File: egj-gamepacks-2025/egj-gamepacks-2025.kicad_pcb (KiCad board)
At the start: 2 copper layers, 52.3 x 64 mm, 81 parts, among them J1 USB_B_Micro, J2 Conn_01x03_Pin, J5 GameBoy_GamePak_AGB-002, SW1 SW_Push, SW2 SW_Push, U1 W25Q128JVS, U10 SP3012-06UTG, U11 VL6180XV0NR_1, U12 TXS0108EPW, U13 LD1117S18TR_SOT223, U14 BNO055, U15 SP3012-06UTG, U2 DNF, U3 NCP1117-3.3_SOT223, U4 RP2350_80QFN, U5 USBLC6-2P6, U6 SP3012-06UTG, U7 SP3012-06UTG, U8 SP3012-06UTG, U9 SP3012-06UTG, Y1 ABM8-272-T3

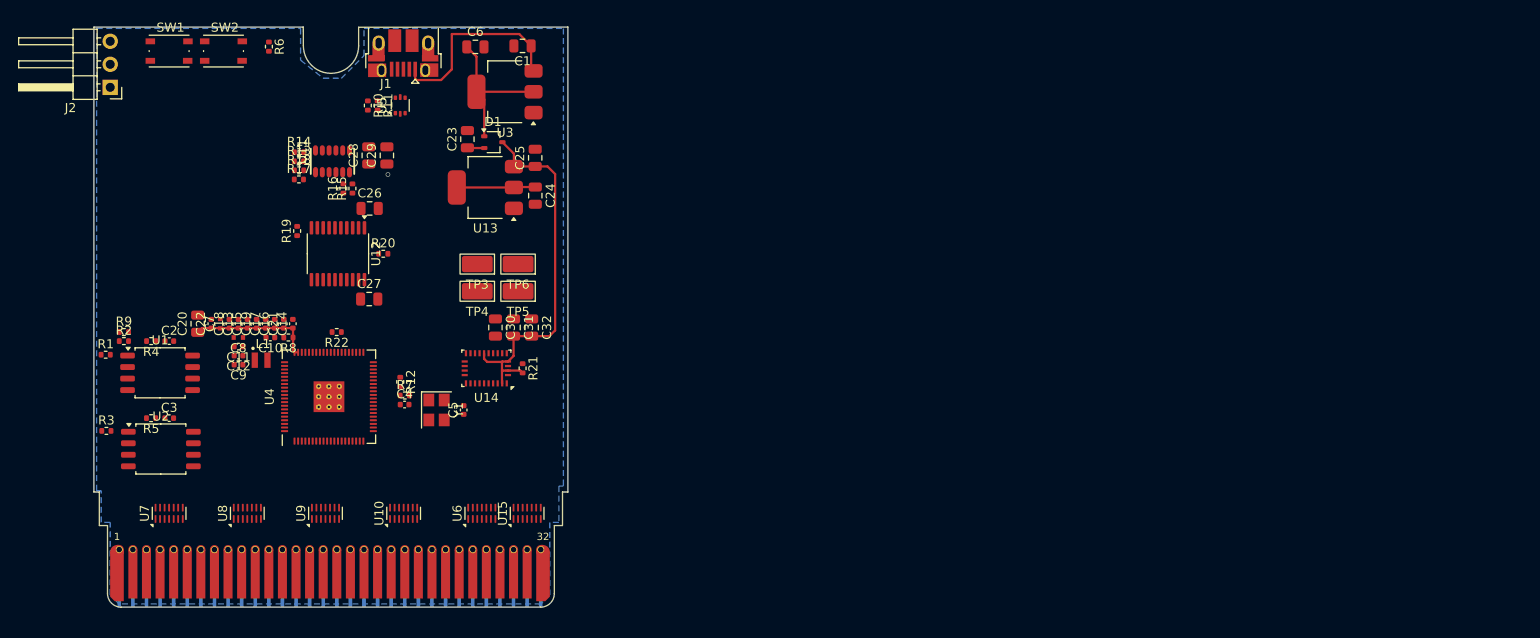
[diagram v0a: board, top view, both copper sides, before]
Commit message: UPDATE: sync local schematic and board work
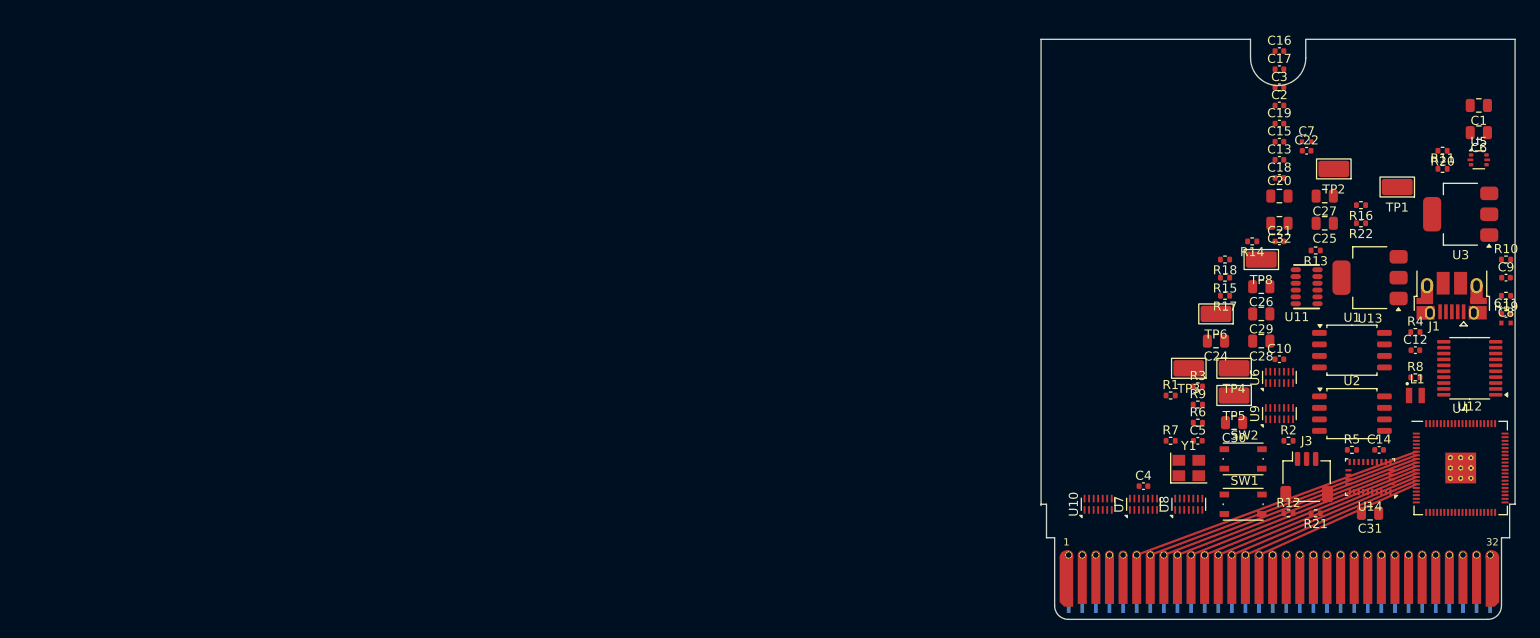
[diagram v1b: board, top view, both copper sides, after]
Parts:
- removed C23: 100u, Capacitor_SMD:C_0805_2012Metric
- removed D1: BAT54CW, Package_TO_SOT_SMD:SOT-323_SC-70
- removed J2: Conn_01x03_Pin, Connector_PinHeader_2.54mm:PinHeader_1x03_P2.54mm_Horizontal
- removed U15: SP3012-06UTG, Package_DFN_QFN:DFN-14_1.35x3.5mm_P0.5mm
- added J3: SM03B-SRSS-TB, Connector_JST:JST_SH_SM03B-SRSS-TB_1x03-1MP_P1.00mm_Horizontal, F.Cu at (251.0, 109.0)
- added TP1: TestPoint, TestPoint:TestPoint_Keystone_5015_Micro_Mini, F.Cu at (261.0, 77.0)
- added TP2: TestPoint, TestPoint:TestPoint_Keystone_5015_Micro_Mini, F.Cu at (254.0, 75.0)
- added TP8: TestPoint, TestPoint:TestPoint_Keystone_5015_Micro_Mini, F.Cu at (246.0, 85.0)
- U13: value LD1117S18TR_SOT223 -> AP7361C-28E
- moved C9 140.2 mm to (273.0, 87.0), turned to 0 degrees
- moved C11 139.9 mm to (273.0, 91.0), turned to 0 degrees
- moved C8 139.9 mm to (273.0, 92.0), turned to 0 degrees
- moved R4 139.5 mm to (263.0, 93.0), turned to 0 degrees
- moved R19 133.6 mm to (273.0, 89.0), turned to 180 degrees
- moved R5 132.5 mm to (256.0, 106.0), turned to 0 degrees
- moved U1 131.5 mm to (256.0, 95.0)
- moved U2 131.5 mm to (256.0, 102.0)
- moved C12 129.8 mm to (263.0, 95.0), turned to 0 degrees
- moved R2 129.0 mm to (249.0, 105.0)
- moved SW1 128.6 mm to (244.0, 112.0)
- moved C3 127.8 mm to (248.0, 66.0)
- moved L1 127.4 mm to (263.0, 100.0)
- moved R10 126.7 mm to (273.0, 85.0), turned to 0 degrees
- moved U12 125.5 mm to (269.0, 97.0), turned to 180 degrees
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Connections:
- net /RP2350/+1V1 renamed +1V1
- C24 pad 1: +1V8 -> +2V8
- C26 pad 1: +1V8 -> +2V8
- C28 pad 1: +1V8 -> +2V8
- C29 pad 1: +1V8 -> +2V8
- C6 pad 1: +3V3_USB -> +3V3
- R10 pad 1: /Power/USB.USB_D_C+ -> /RP2350/USB_D+
- R11 pad 1: /Power/USB.USB_D_C- -> /RP2350/USB_D-
- R13 pad 1: +1V8 -> +2V8
- R14 pad 1: +1V8 -> +2V8
- R17 pad 1: +1V8 -> +2V8
- R18 pad 1: +1V8 -> +2V8
- U10 pad 1: /GBA_Connector/GBA_ADD13 -> unconnected-(U10-Pad1)
- U10 pad 11: /GBA_Connector/GBA_DATA0 -> /GBA_Connector/GBA_SIG.N_CS
- U10 pad 12: /GBA_Connector/GBA_ADD15 -> /GBA_Connector/GBA_SIG.N_RD
- U10 pad 13: /GBA_Connector/GBA_ADD14 -> /GBA_Connector/GBA_SIG.N_WR
- U10 pad 14: /GBA_Connector/GBA_ADD13 -> /GBA_Connector/GBA_SIG.PHI
- U10 pad 2: /GBA_Connector/GBA_ADD14 -> unconnected-(U10-Pad2)
- U10 pad 3: /GBA_Connector/GBA_ADD15 -> unconnected-(U10-Pad3)
- U10 pad 4: /GBA_Connector/GBA_DATA0 -> unconnected-(U10-Pad4)
- U10 pad 5: GND -> unconnected-(U10-Pad5)
- U10 pad 6: /GBA_Connector/GBA_DATA1 -> unconnected-(U10-Pad6)
- U10 pad 7: /GBA_Connector/GBA_DATA2 -> unconnected-(U10-Pad7)
- U10 pad 8: /GBA_Connector/GBA_DATA2 -> /GBA_Connector/GBA_SIG.IRQ
- U10 pad 9: /GBA_Connector/GBA_DATA1 -> /GBA_Connector/GBA_SIG.N_CS2
- U11 pad 10: +1V8 -> +2V8
- U11 pad 8: +1V8 -> +2V8
- U12 pad 2: +1V8 -> +2V8
- U13 pad 1: GND -> +3V3
- U13 pad 2: +1V8 -> GND
- U13 pad 3: +3V3 -> +2V8
- U3 pad 2: +3V3_USB -> +3V3
- U4 pad 1: /GBA_Connector/GBA_ADD0 -> /GBA_Connector/GBA_DATA4
- U4 pad 11: /GBA_Connector/GBA_ADD8 -> /GBA_Connector/GBA_ADD4
- U4 pad 12: /GBA_Connector/GBA_ADD9 -> /GBA_Connector/GBA_ADD5
- U4 pad 13: /GBA_Connector/GBA_ADD10 -> /GBA_Connector/GBA_ADD6
- U4 pad 14: /GBA_Connector/GBA_ADD11 -> /GBA_Connector/GBA_ADD7
- U4 pad 16: /GBA_Connector/GBA_ADD12 -> /GBA_Connector/GBA_ADD8
- U4 pad 17: /GBA_Connector/GBA_ADD13 -> /GBA_Connector/GBA_ADD9
- U4 pad 18: /GBA_Connector/GBA_ADD14 -> /GBA_Connector/GBA_ADD10
- U4 pad 19: /GBA_Connector/GBA_ADD15 -> /GBA_Connector/GBA_ADD11
- U4 pad 2: /GBA_Connector/GBA_ADD1 -> /GBA_Connector/GBA_DATA5
- U4 pad 20: /GBA_Connector/GBA_DATA0 -> /GBA_Connector/GBA_ADD12
- U4 pad 21: /GBA_Connector/GBA_DATA1 -> /GBA_Connector/GBA_ADD13
- U4 pad 22: /GBA_Connector/GBA_DATA2 -> /GBA_Connector/GBA_ADD14
- U4 pad 23: /GBA_Connector/GBA_DATA3 -> /GBA_Connector/GBA_ADD15
- U4 pad 25: /GBA_Connector/GBA_DATA4 -> /GBA_Connector/GBA_SIG.PHI
- U4 pad 26: /GBA_Connector/GBA_DATA5 -> /GBA_Connector/GBA_SIG.N_WR
- U4 pad 27: /GBA_Connector/GBA_DATA6 -> /GBA_Connector/GBA_SIG.N_RD
- U4 pad 28: /GBA_Connector/GBA_DATA7 -> /GBA_Connector/GBA_SIG.N_CS
- U4 pad 3: /GBA_Connector/GBA_ADD2 -> /GBA_Connector/GBA_DATA6
- U4 pad 4: /GBA_Connector/GBA_ADD3 -> /GBA_Connector/GBA_DATA7
- U4 pad 58: +3V3_USB -> unconnected-(U4-GPIO47_ADC7-Pad58)
- U4 pad 6: /GBA_Connector/GBA_ADD4 -> /GBA_Connector/GBA_ADD0
- U4 pad 7: /GBA_Connector/GBA_ADD5 -> /GBA_Connector/GBA_ADD1
- U4 pad 77: /GBA_Connector/GBA_SIG.PHI -> /GBA_Connector/GBA_DATA0
- U4 pad 78: /GBA_Connector/GBA_SIG.N_WR -> /GBA_Connector/GBA_DATA1
- U4 pad 79: /GBA_Connector/GBA_SIG.N_RD -> /GBA_Connector/GBA_DATA2
- U4 pad 8: /GBA_Connector/GBA_ADD6 -> /GBA_Connector/GBA_ADD2
- U4 pad 80: /GBA_Connector/GBA_SIG.N_CS -> /GBA_Connector/GBA_DATA3
- U4 pad 9: /GBA_Connector/GBA_ADD7 -> /GBA_Connector/GBA_ADD3
- U5 pad 2: unconnected-(U5-GND-Pad2) -> GND
- U5 pad 4: /Power/USB.USB_D_C- -> /RP2350/USB_D-
- U5 pad 5: GND -> VBUS
- U5 pad 6: /Power/USB.USB_D_C+ -> /RP2350/USB_D+
- U6 pad 1: /GBA_Connector/GBA_DATA3 -> unconnected-(U6-Pad1)
- U6 pad 11: /GBA_Connector/GBA_DATA6 -> /GBA_Connector/GBA_DATA3
- U6 pad 12: /GBA_Connector/GBA_DATA5 -> /GBA_Connector/GBA_DATA2
- U6 pad 13: /GBA_Connector/GBA_DATA4 -> /GBA_Connector/GBA_DATA1
- U6 pad 14: /GBA_Connector/GBA_DATA3 -> /GBA_Connector/GBA_DATA0
- U6 pad 2: /GBA_Connector/GBA_DATA4 -> unconnected-(U6-Pad2)
- U6 pad 3: /GBA_Connector/GBA_DATA5 -> unconnected-(U6-Pad3)
- U6 pad 4: /GBA_Connector/GBA_DATA6 -> unconnected-(U6-Pad4)
- U6 pad 5: GND -> unconnected-(U6-Pad5)
- U6 pad 6: /GBA_Connector/GBA_DATA7 -> unconnected-(U6-Pad6)
- U6 pad 7: /GBA_Connector/GBA_SIG.N_CS2 -> unconnected-(U6-Pad7)
- U6 pad 8: /GBA_Connector/GBA_SIG.N_CS2 -> /GBA_Connector/GBA_DATA5
- U6 pad 9: /GBA_Connector/GBA_DATA7 -> /GBA_Connector/GBA_DATA4
- U7 pad 1: /GBA_Connector/GBA_SIG.PHI -> unconnected-(U7-Pad1)
- U7 pad 11: /GBA_Connector/GBA_SIG.N_CS -> /GBA_Connector/GBA_ADD1
- U7 pad 12: /GBA_Connector/GBA_SIG.N_RD -> /GBA_Connector/GBA_ADD0
- U7 pad 13: /GBA_Connector/GBA_SIG.N_WR -> /GBA_Connector/GBA_DATA7
- U7 pad 14: /GBA_Connector/GBA_SIG.PHI -> /GBA_Connector/GBA_DATA6
- U7 pad 2: /GBA_Connector/GBA_SIG.N_WR -> unconnected-(U7-Pad2)
- U7 pad 3: /GBA_Connector/GBA_SIG.N_RD -> unconnected-(U7-Pad3)
- U7 pad 4: /GBA_Connector/GBA_SIG.N_CS -> unconnected-(U7-Pad4)
- U7 pad 5: GND -> unconnected-(U7-Pad5)
- U7 pad 6: /GBA_Connector/GBA_ADD0 -> unconnected-(U7-Pad6)
- U7 pad 7: /GBA_Connector/GBA_ADD1 -> unconnected-(U7-Pad7)
- U7 pad 8: /GBA_Connector/GBA_ADD1 -> /GBA_Connector/GBA_ADD3
- U7 pad 9: /GBA_Connector/GBA_ADD0 -> /GBA_Connector/GBA_ADD2
- U8 pad 1: /GBA_Connector/GBA_ADD2 -> unconnected-(U8-Pad1)
- U8 pad 11: /GBA_Connector/GBA_ADD4 -> /GBA_Connector/GBA_ADD7
- U8 pad 12: /GBA_Connector/GBA_ADD3 -> /GBA_Connector/GBA_ADD6
- U8 pad 13: /GBA_Connector/GBA_ADD2 -> /GBA_Connector/GBA_ADD5
- U8 pad 14: /GBA_Connector/GBA_ADD2 -> /GBA_Connector/GBA_ADD4
- U8 pad 2: /GBA_Connector/GBA_ADD2 -> unconnected-(U8-Pad2)
- U8 pad 3: /GBA_Connector/GBA_ADD3 -> unconnected-(U8-Pad3)
- U8 pad 4: /GBA_Connector/GBA_ADD4 -> unconnected-(U8-Pad4)
- U8 pad 5: GND -> unconnected-(U8-Pad5)
- U8 pad 6: /GBA_Connector/GBA_ADD5 -> unconnected-(U8-Pad6)
- U8 pad 7: /GBA_Connector/GBA_ADD6 -> unconnected-(U8-Pad7)
- U8 pad 8: /GBA_Connector/GBA_ADD6 -> /GBA_Connector/GBA_ADD9
- U8 pad 9: /GBA_Connector/GBA_ADD5 -> /GBA_Connector/GBA_ADD8
- U9 pad 1: /GBA_Connector/GBA_ADD7 -> unconnected-(U9-Pad1)
- U9 pad 11: /GBA_Connector/GBA_ADD10 -> /GBA_Connector/GBA_ADD13
- U9 pad 12: /GBA_Connector/GBA_ADD9 -> /GBA_Connector/GBA_ADD12
- U9 pad 13: /GBA_Connector/GBA_ADD8 -> /GBA_Connector/GBA_ADD11
- U9 pad 14: /GBA_Connector/GBA_ADD7 -> /GBA_Connector/GBA_ADD10
- U9 pad 2: /GBA_Connector/GBA_ADD8 -> unconnected-(U9-Pad2)
- U9 pad 3: /GBA_Connector/GBA_ADD9 -> unconnected-(U9-Pad3)
- U9 pad 4: /GBA_Connector/GBA_ADD10 -> unconnected-(U9-Pad4)
- U9 pad 5: GND -> unconnected-(U9-Pad5)
- U9 pad 6: /GBA_Connector/GBA_ADD11 -> unconnected-(U9-Pad6)
- U9 pad 7: /GBA_Connector/GBA_ADD12 -> unconnected-(U9-Pad7)
- U9 pad 8: /GBA_Connector/GBA_ADD12 -> /GBA_Connector/GBA_ADD15
- U9 pad 9: /GBA_Connector/GBA_ADD11 -> /GBA_Connector/GBA_ADD14
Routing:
- net +3V3: track 55.3 -> 0.00 mm
- net /GBA_Connector/GBA_ADD0: track 0.00 -> 32.9 mm
- net /GBA_Connector/GBA_ADD1: track 0.00 -> 31.3 mm
- net /GBA_Connector/GBA_ADD2: track 0.00 -> 29.8 mm
- net /GBA_Connector/GBA_ADD3: track 0.00 -> 28.3 mm
- net /GBA_Connector/GBA_ADD4: track 0.00 -> 26.7 mm
- net /GBA_Connector/GBA_ADD5: track 0.00 -> 25.2 mm
- net /GBA_Connector/GBA_ADD6: track 0.00 -> 23.6 mm
- net /GBA_Connector/GBA_ADD7: track 0.00 -> 22.1 mm
- net VBUS: track 21.7 -> 0.00 mm
- net /GBA_Connector/GBA_ADD8: track 0.00 -> 20.6 mm
- net /GBA_Connector/GBA_ADD9: track 0.00 -> 19.0 mm
- net +3V3_USB: track 17.0 -> 0.00 mm
- net +1V8: track 8.68 -> 0.00 mm
- net +3V3_GBA: track 1.87 -> 0.00 mm
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- removed copper zone on B.Cu, net (none)
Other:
- outline, holes or cut-outs redrawn
